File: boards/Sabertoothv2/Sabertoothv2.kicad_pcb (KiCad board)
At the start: 2 copper layers, 50 x 50 mm, 29 parts, among them J1 Screw_Terminal_01x04, J2 Screw_Terminal_01x04, J3 Conn_01x04_Pin, J4 Conn_01x04_Pin, Q1 NMOS, Q2 NMOS, Q3 NMOS, Q4 NMOS, U1 LM2104, U2 LM2104, U3 74LVC1GU04DRL

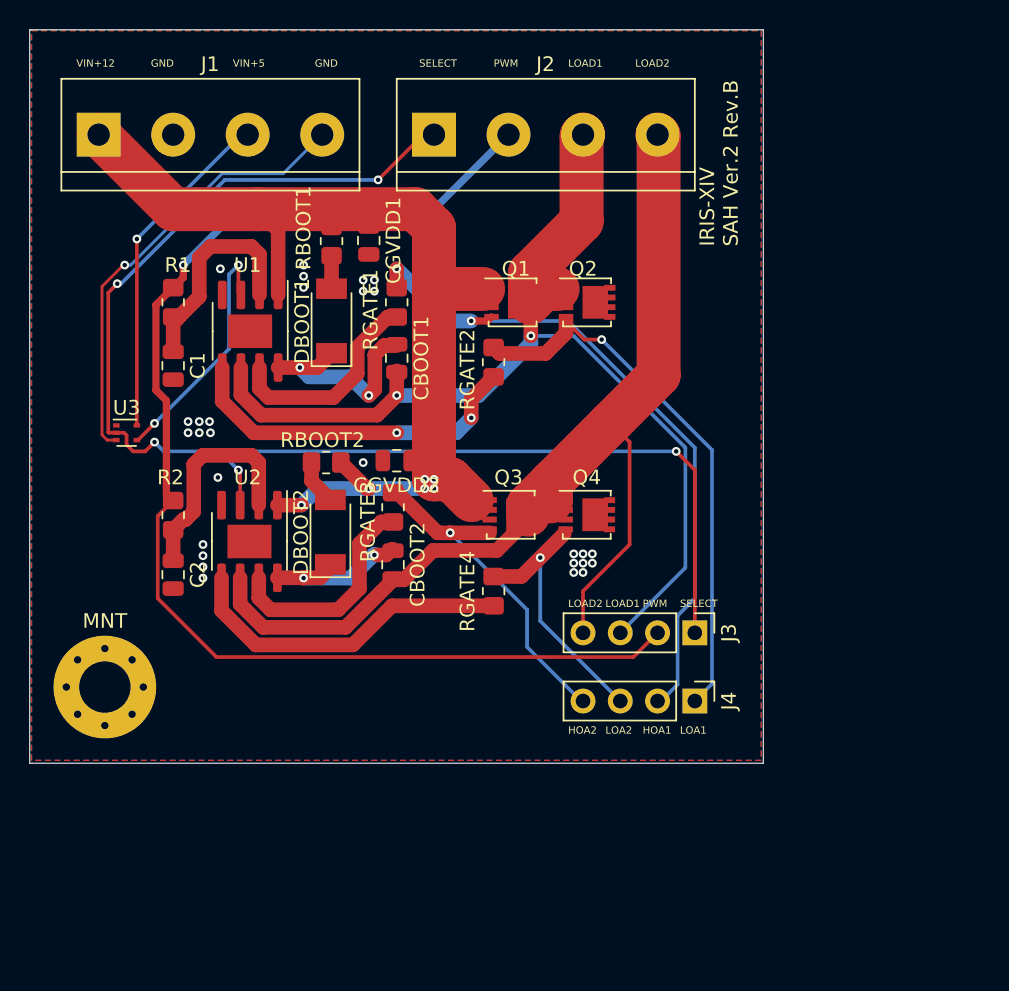
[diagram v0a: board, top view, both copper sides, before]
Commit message: changing pcb
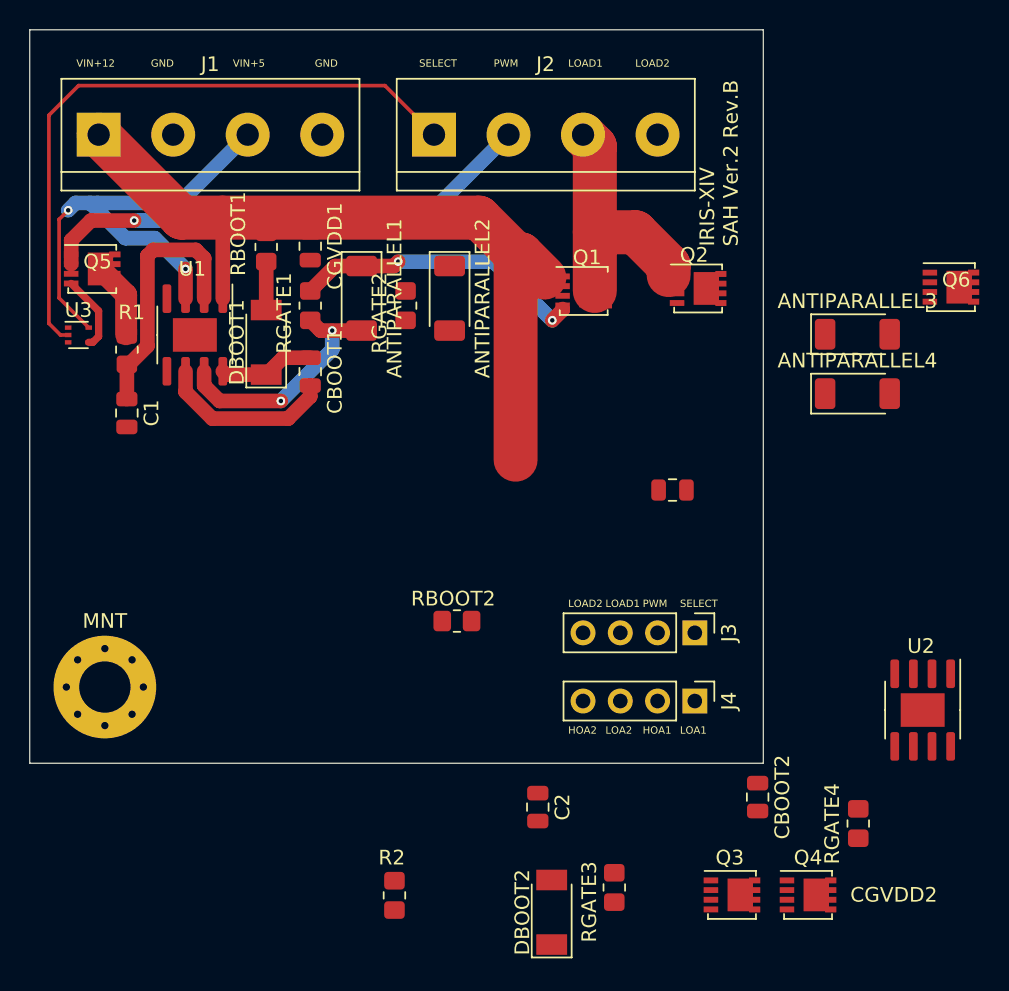
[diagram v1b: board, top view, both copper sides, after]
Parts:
- added ANTIPARALLEL1: 1V, Diode_SMD:D_SOD-128, F.Cu at (52.5, 48.5)
- added ANTIPARALLEL2: 1V, Diode_SMD:D_SOD-128, F.Cu at (58.5, 48.5)
- added ANTIPARALLEL3: 1V, Diode_SMD:D_SOD-128, F.Cu at (86.3, 51.0)
- added ANTIPARALLEL4: 1V, Diode_SMD:D_SOD-128, F.Cu at (86.3, 55.0)
- added Q5: NMOS, mosfet:PPAK1212-8Custom, F.Cu at (34.5, 46.5)
- added Q6: NMOS, mosfet:PPAK1212-8Custom, F.Cu at (93.0, 47.7)
- moved U2 47.3 mm to (90.8, 76.6)
- moved RGATE3 30.0 mm to (69.7, 88.7)
- moved DBOOT2 30.0 mm to (65.5, 90.4)
- moved Q4 30.0 mm to (83.3, 89.2)
- moved R2 30.0 mm to (54.7, 89.2)
- moved Q3 30.0 mm to (78.1, 89.2)
- moved RGATE4 29.5 mm to (86.4, 84.3)
- moved C2 29.5 mm to (64.5, 83.2)
- moved CBOOT2 29.5 mm to (79.5, 82.5)
- moved CGVDD2 18.9 mm to (73.7, 61.6)
- moved RBOOT2 14.0 mm to (59.0, 70.5)
- moved Q2 7.63 mm to (75.8, 47.8)
- moved U3 7.43 mm to (33.2, 51.0)
- moved RGATE2 7.13 mm to (55.5, 49.0)
- moved CBOOT1 5.97 mm to (49.0, 53.5)
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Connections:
- J4 pad 1: LOA -> VIN+12
- J4 pad 2: HOA -> GND
- J4 pad 3: LOB -> LOA
- J4 pad 4: HOB -> HOA
- R1 pad 1: PWM -> Net-(Q5-S)
- R2 pad 1: PWM -> Net-(Q6-S)
- U1 pad 3: Net-(U1-SD') -> VIN+5
- U2 pad 3: SELECT -> VIN+5
- U3 pad 3: LGND -> GND
- U3 pad 4: Net-(U1-SD') -> Net-(Q5-G)
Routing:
- net LOAD2: track 72.2 -> 0.00 mm
- net PWM: track 86.7 -> 34.4 mm
- net SELECT: track 93.5 -> 44.3 mm, vias 5 -> 0
- net LOAD1: track 72.1 -> 29.6 mm, vias 2 -> 0
- net LOA: track 37.7 -> 0.00 mm, vias 1 -> 0
- net LGND: track 30.5 -> 0.00 mm, vias 1 -> 0
- net HOA: track 46.6 -> 20.0 mm
- net Net-(ANTIPARALLEL2-A): track 24.0 -> 0.00 mm, vias 2 -> 0
- net HOB: track 23.0 -> 0.00 mm, vias 1 -> 0
- net Net-(ANTIPARALLEL4-A): track 22.9 -> 0.00 mm
- net LOB: track 18.1 -> 0.00 mm, vias 1 -> 0
- net VIN+12: track 71.6 -> 54.0 mm, vias 6 -> 0
- net Net-(U1-SD'): track 16.9 -> 0.00 mm, vias 2 -> 0
- net Net-(ANTIPARALLEL3-A): track 15.1 -> 0.00 mm
- net Net-(U2-IN): track 15.0 -> 0.00 mm
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- removed copper zone on B.Cu, net GND
- removed copper zone on F.Cu, net GND
